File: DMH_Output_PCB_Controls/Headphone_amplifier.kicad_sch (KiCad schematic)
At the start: 24 parts, among them U11 TL074, U12 NE5532, U13 NE5532, U14 NE5532, U15 NE5532

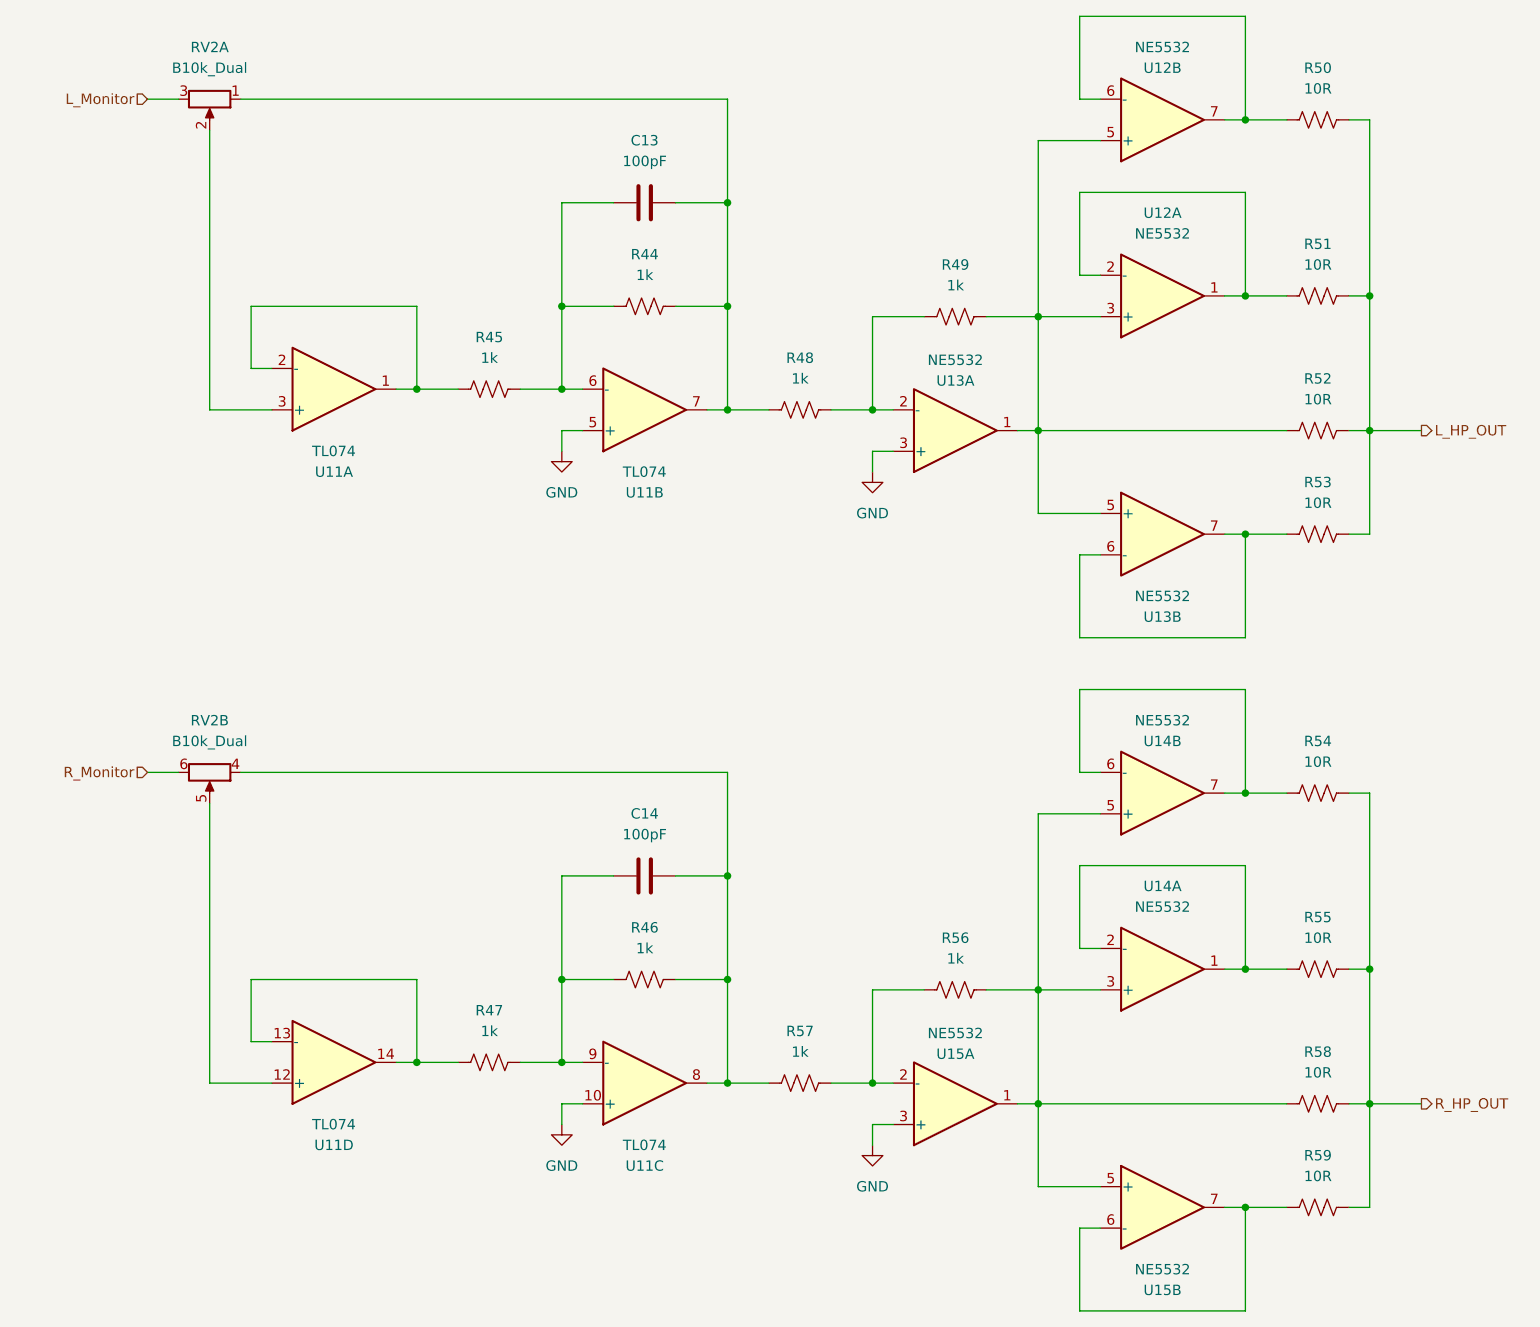
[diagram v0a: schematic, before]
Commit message: Starting Controls PCB design
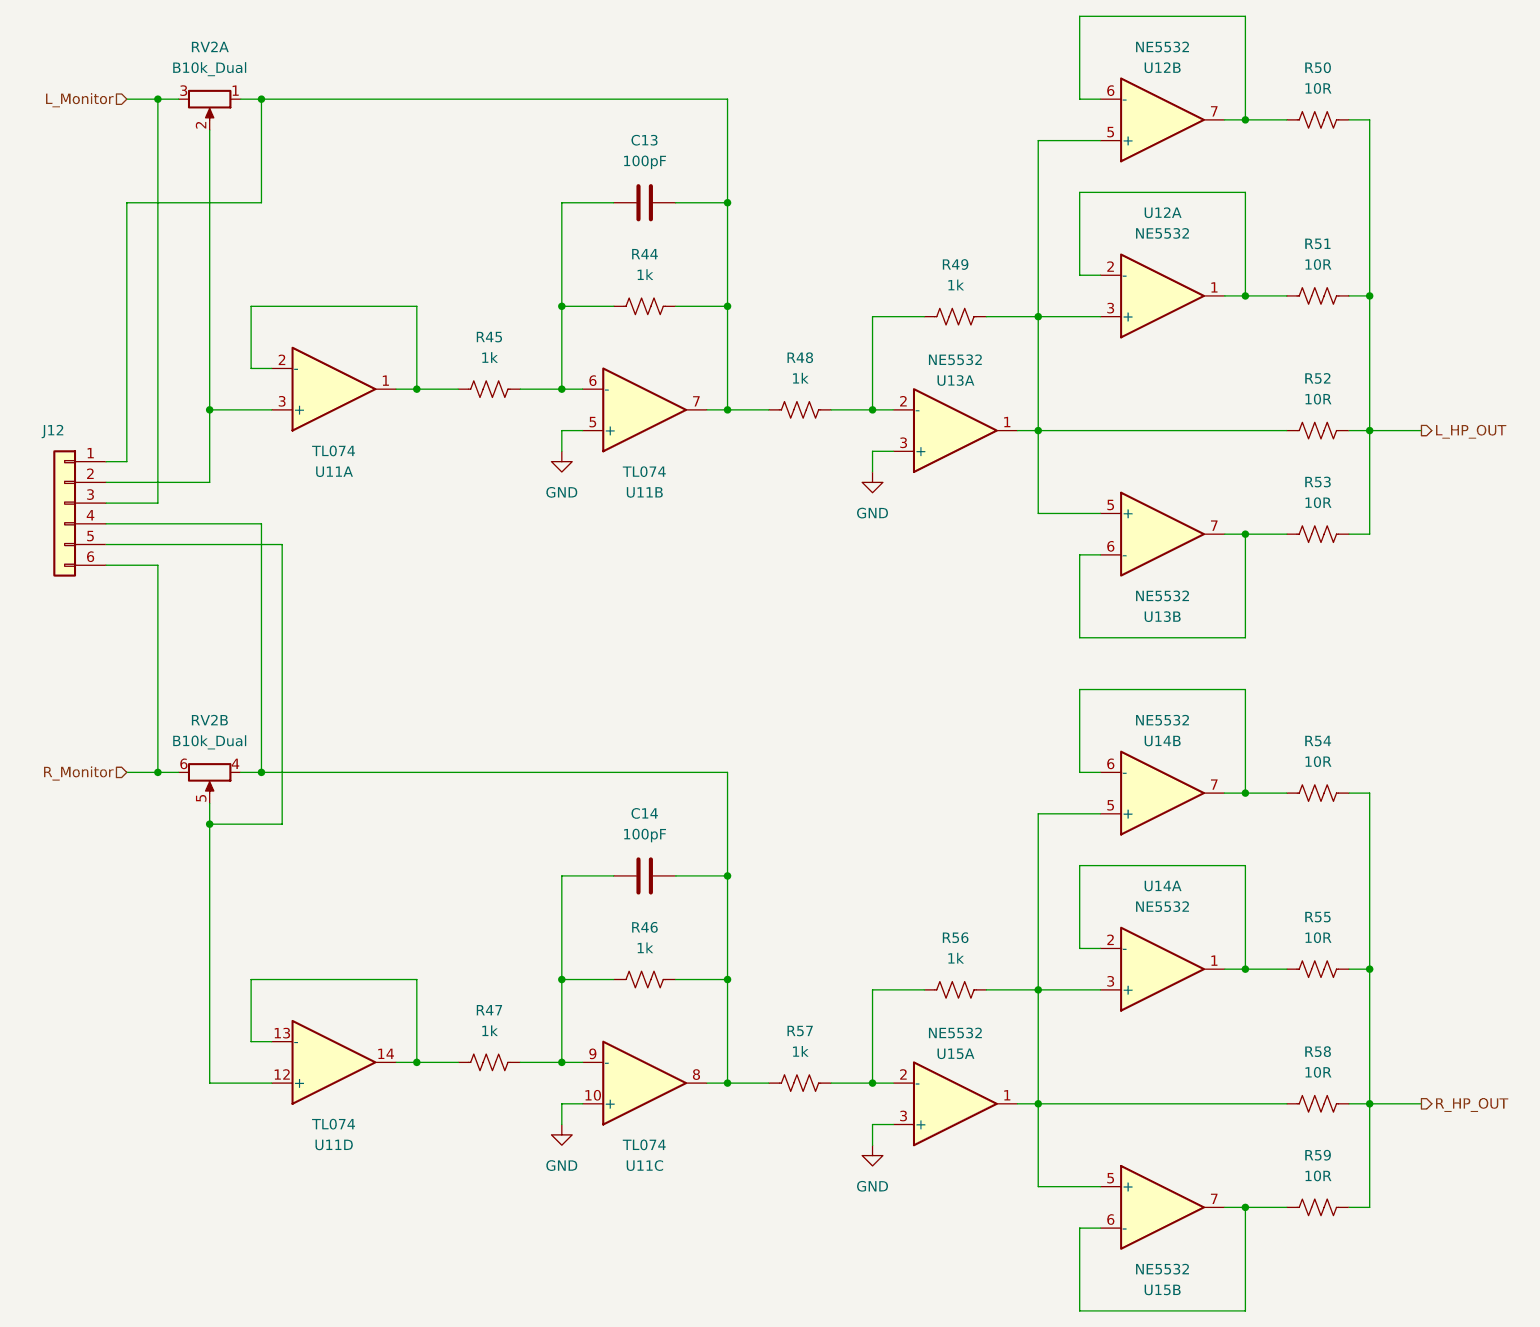
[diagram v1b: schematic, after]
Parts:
- added J12: Conn_01x06, Connector_PinSocket_2.54mm:PinSocket_1x06_P2.54mm_Vertical, symbol Connector_Generic:Conn_01x06
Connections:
- net L_Monitor: now also J12.3 (Pin_3)
- net R_Monitor: now also J12.6 (Pin_6)
- net at RV2.5, U11.12 (+): now also J12.5 (Pin_5)
- net at C13.2, R44.2, R48.1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: now also J12.1 (Pin_1)
- net at RV2.2, U11.3 (+): now also J12.2 (Pin_2)
- net at C14.2, R46.2, R57.1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: now also J12.4 (Pin_4)
